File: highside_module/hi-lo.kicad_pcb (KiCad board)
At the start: 2 copper layers, 43.4 x 20.3 mm, 31 parts, among them M601 CONN_1, P601 CONN_3X2, P602 CONN_2, P603 CONN_6, P604 CONN_2, P606 CONN_2, U601 TC4427, U602 TC4427, U603 TC4427

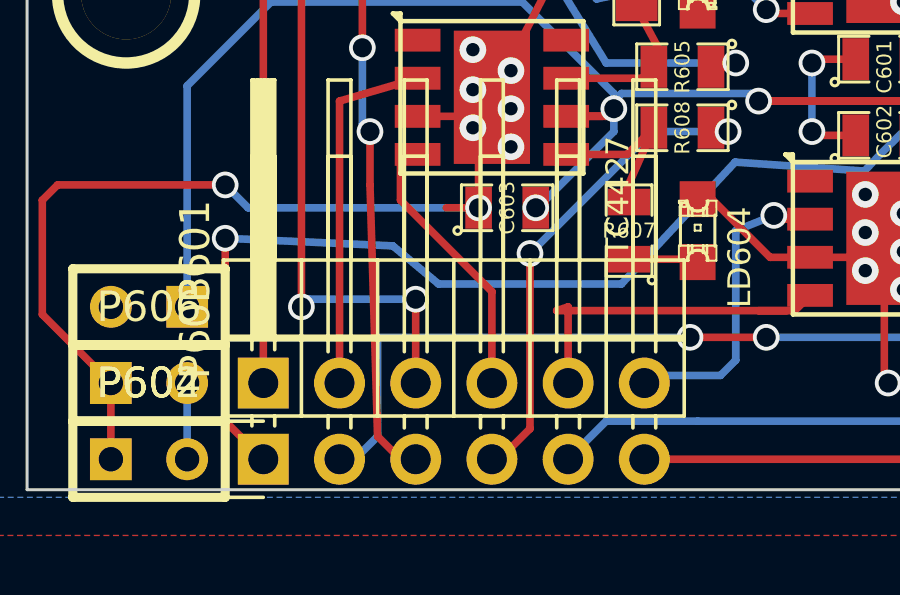
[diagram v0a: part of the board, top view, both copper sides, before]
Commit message: silkscreen
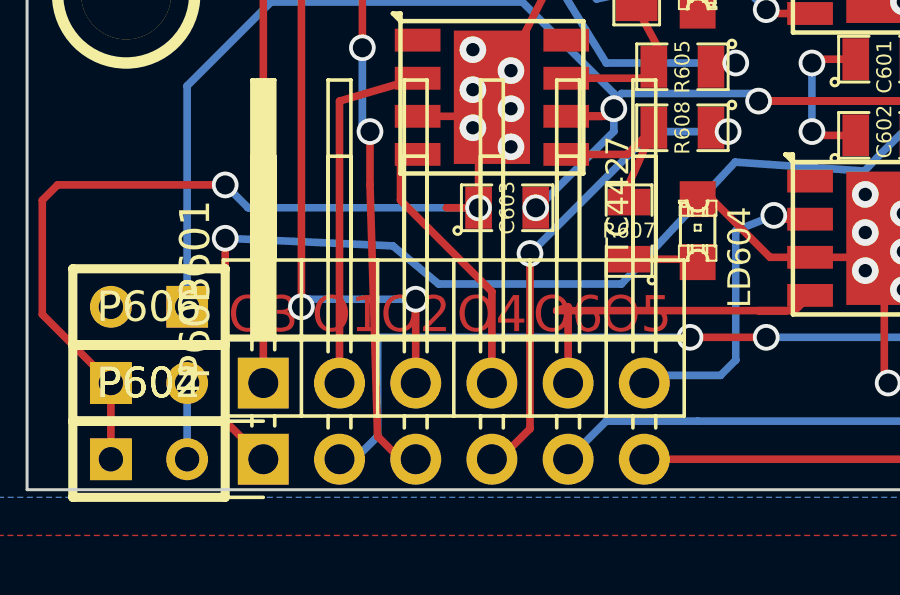
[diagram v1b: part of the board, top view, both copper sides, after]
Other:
- board text added: "O1"
- board text added: "O2"
- board text added: "O3"
- board text added: "O4"
- board text added: "O5"
- board text added: "O6"
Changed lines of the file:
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@@
-(kicad_pcb (version 4) (host pcbnew 4.0.7)
+(kicad_pcb (version 4) (host pcbnew 4.0.1-stable)
   (general
     (links 53)
     (no_connects 0)
-    (area 28.778999 12.121499 247.169715 255.053501)
+    (area 28.778999 12.121499 247.319715 255.053501)
     (thickness 1.6)
-    (drawings 51)
+    (drawings 57)
     (tracks 317)
     (zones 0)
@@
     )
   )
+  (gr_text O5 (at 195.326 162.814) (layer F.Cu)
+    (effects (font (size 1.2 1.2) (thickness 0.3)))
+  )
+  (gr_text O6 (at 193.04 162.814) (layer F.Cu)
+    (effects (font (size 1.2 1.2) (thickness 0.3)))
+  )
+  (gr_text O4 (at 190.5 162.814) (layer F.Cu)
+    (effects (font (size 1.2 1.2) (thickness 0.3)))
+  )
+  (gr_text O3 (at 182.88 162.814) (layer F.Cu)
+    (effects (font (size 1.2 1.2) (thickness 0.3)))
+  )
+  (gr_text O2 (at 187.96 162.814) (layer F.Cu)
+    (effects (font (size 1.2 1.2) (thickness 0.3)))
+  )
+  (gr_text O1 (at 185.674 162.814) (layer F.Cu)
+    (effects (font (size 1.2 1.2) (thickness 0.3)))
+  )
   (dimension 20.32 (width 0.3) (layer Cmts.User)
